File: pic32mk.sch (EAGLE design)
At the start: 85 parts, among them IC1 PIC32MK1024MCF100-I_PT, IC2 ADM3095EBRZ, IC3 TXB0101DCKR, IC4 MAX203ECWP, IC5 TXB0101DCKR, IC6 TXB0101DCKR, IC7 TXB0101DCKR, IC8 TXB0101DCKR, IC9 TXB0101DCKR, J1 1-1586043-4, U1 PMIC-MC33932VW(SOP44), U2 PMIC-MC33932VW(SOP44), U3 ULN2803ADW, U4 REF3440IDBVR, X1 22-23-2101, X2 22-23-2081

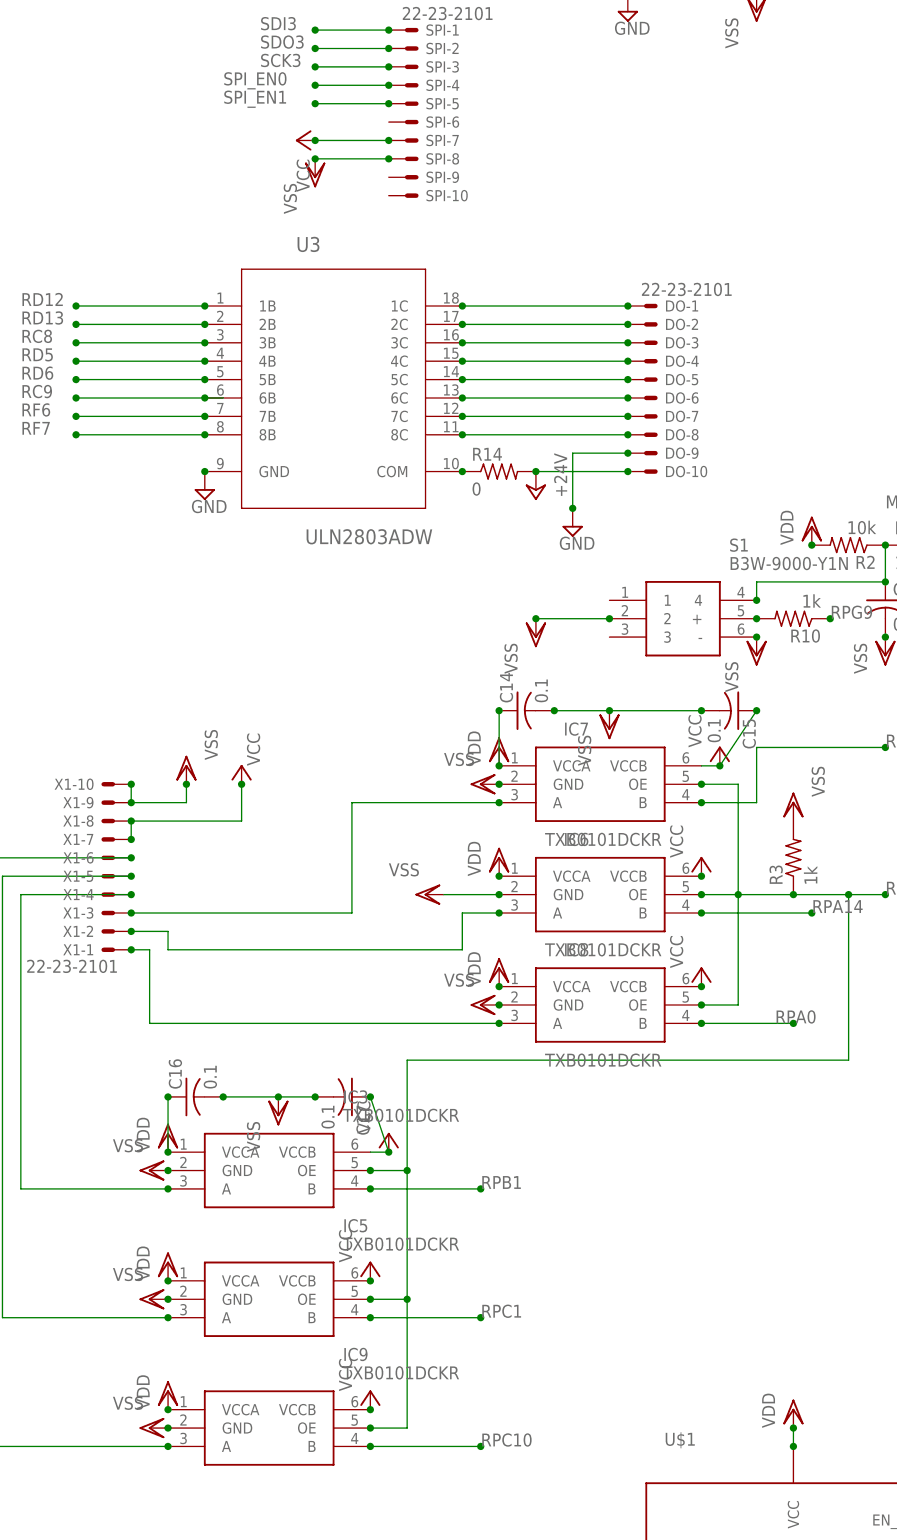
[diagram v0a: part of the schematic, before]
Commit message: up
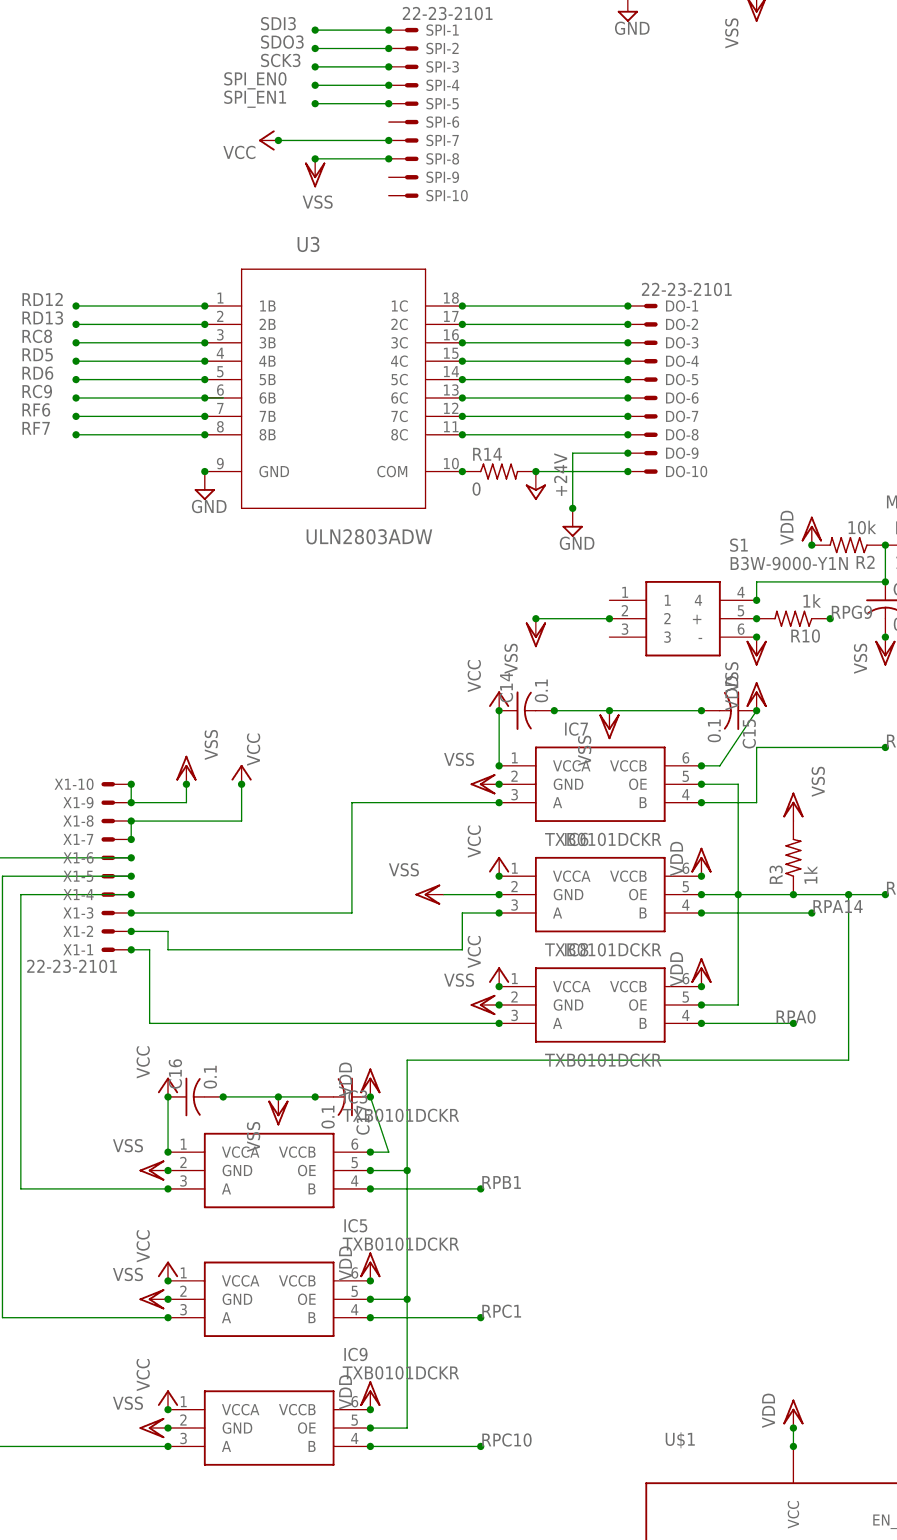
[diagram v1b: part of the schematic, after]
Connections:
- net VCC: now also C14.1, C16.1, IC3.VCCA, IC5.VCCA, IC6.VCCA, IC7.VCCA, IC8.VCCA, IC9.VCCA; no longer C15.1, C17.1, IC3.VCCB, IC5.VCCB, IC6.VCCB, IC7.VCCB, IC8.VCCB, IC9.VCCB
- net VDD: now also C15.1, C17.1, IC3.VCCB, IC5.VCCB, IC6.VCCB, IC7.VCCB, IC8.VCCB, IC9.VCCB; no longer C14.1, C16.1, IC3.VCCA, IC5.VCCA, IC6.VCCA, IC7.VCCA, IC8.VCCA, IC9.VCCA

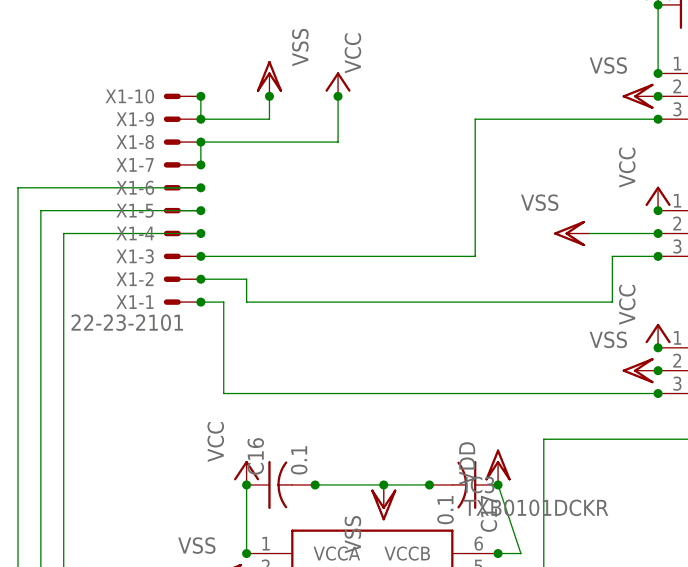
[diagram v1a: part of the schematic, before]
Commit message: up
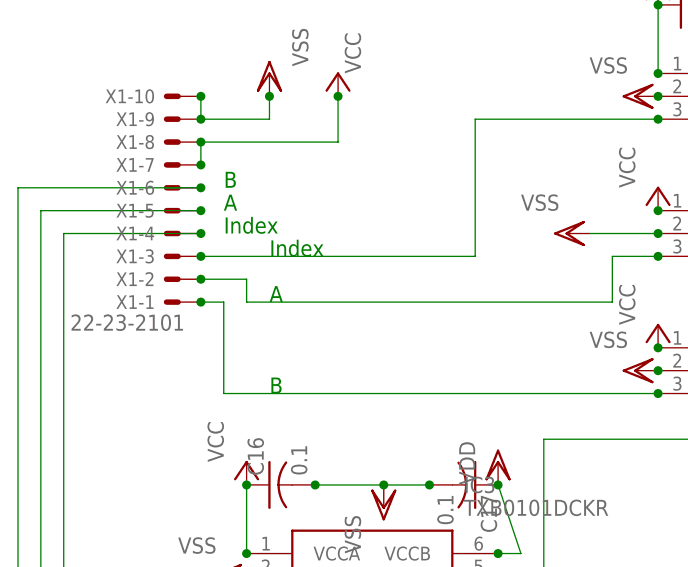
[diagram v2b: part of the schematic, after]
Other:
- note added: "A"
- note added: "B"
- note added: "Index"
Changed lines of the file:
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@@
 <text x="-12.7" y="-109.22" size="1.778" layer="91">change to VDD from VSS</text>
 <text x="-12.7" y="-86.36" size="1.778" layer="91">change to VSS from orig VCC</text>
+<text x="-132.08" y="-40.64" size="1.778" layer="91">A</text>
+<text x="-132.08" y="-50.8" size="1.778" layer="91">B</text>
+<text x="-132.08" y="-35.56" size="1.778" layer="91">Index</text>
+<text x="-137.16" y="-33.02" size="1.778" layer="91">Index</text>
+<text x="-137.16" y="-30.48" size="1.778" layer="91">A</text>
+<text x="-137.16" y="-27.94" size="1.778" layer="91">B</text>
 </plain>
 <instances>
